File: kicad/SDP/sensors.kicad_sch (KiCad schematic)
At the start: 13 parts, among them J10 Limit, J11 Conn_01x07, J12 Conn_01x07, J13 Conn_01x03, J14 Conn_01x03, J8 Conn_01x07, J9 Conn_01x07

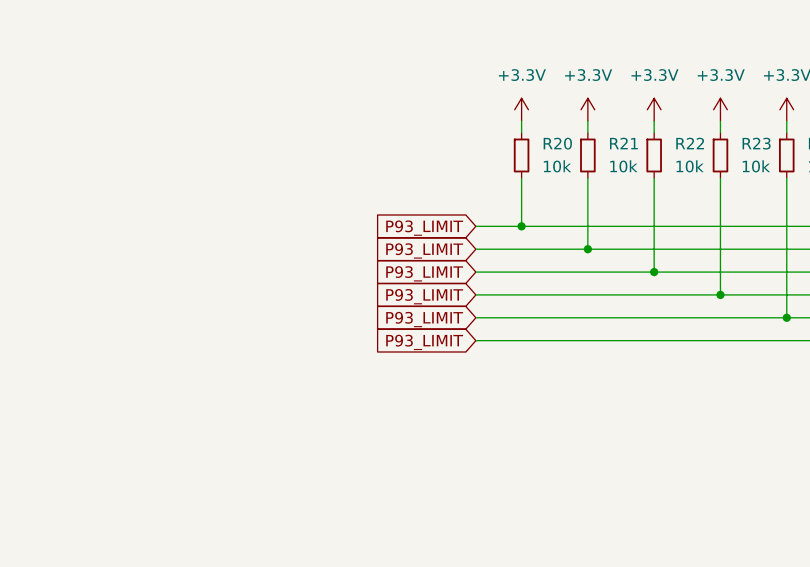
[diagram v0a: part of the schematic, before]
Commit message: PCB layout and schematic updates
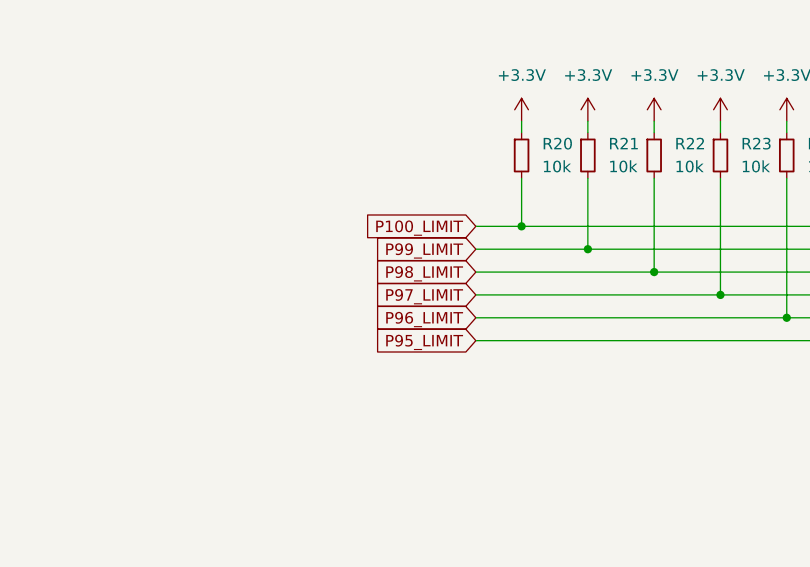
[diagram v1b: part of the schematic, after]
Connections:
- removed net P93_LIMIT: J10.1 (Pin_1), J10.11 (Pin_11), J10.3 (Pin_3), J10.5 (Pin_5), J10.7 (Pin_7), J10.9 (Pin_9), R20.2, R21.2, R22.2, R23.2, R24.2, R25.2
- new net P100_LIMIT: J10.1 (Pin_1), R20.2
- new net P95_LIMIT: J10.11 (Pin_11), R25.2
- new net P96_LIMIT: J10.9 (Pin_9), R24.2
- new net P97_LIMIT: J10.7 (Pin_7), R23.2
- new net P98_LIMIT: J10.5 (Pin_5), R22.2
- new net P99_LIMIT: J10.3 (Pin_3), R21.2
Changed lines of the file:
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@@
     (effects (font (size 1.27 1.27)) (justify left bottom))
+  )
+  (global_label "P100_LIMIT" (shape input) (at 179.832 53.086 180) (fields_autoplaced)
+    (effects (font (size 1.27 1.27)) (justify right))
+    (property "Intersheet References" "${INTERSHEET_REFS}" (id 0) (at 166.896 53.1654 0)
+      (effects (font (size 1.27 1.27)) (justify right) hide)
+    )
   )
   (global_label "P57_SCL1" (shape input) (at 91.694 39.116 180) (fields_autoplaced)
@@
     (effects (font (size 1.27 1.27)) (justify right))
     (property "Intersheet References" "${INTERSHEET_REFS}" (id 0) (at 73.3757 44.1166 0)
-      (effects (font (size 1.27 1.27)) (justify right) hide)
-    )
-  )
-  (global_label "P93_LIMIT" (shape input) (at 179.832 60.706 180) (fields_autoplaced)
-    (effects (font (size 1.27 1.27)) (justify right))
-    (property "Intersheet References" "${INTERSHEET_REFS}" (id 0) (at 168.1056 60.6266 0)
       (effects (font (size 1.27 1.27)) (justify right) hide)
     )
@@
     )
   )
+  (global_label "P95_LIMIT" (shape input) (at 179.832 65.786 180) (fields_autoplaced)
+    (effects (font (size 1.27 1.27)) (justify right))
+    (property "Intersheet References" "${INTERSHEET_REFS}" (id 0) (at 168.1056 65.7066 0)
+      (effects (font (size 1.27 1.27)) (justify right) hide)
+    )
+  )
   (global_label "P56_SDA1" (shape input) (at 91.694 36.576 180) (fields_autoplaced)
     (effects (font (size 1.27 1.27)) (justify right))
     (property "Intersheet References" "${INTERSHEET_REFS}" (id 0) (at 79.8466 36.4966 0)
+      (effects (font (size 1.27 1.27)) (justify right) hide)
+    )
+  )
+  (global_label "P97_LIMIT" (shape input) (at 179.832 60.706 180) (fields_autoplaced)
+    (effects (font (size 1.27 1.27)) (justify right))
+    (property "Intersheet References" "${INTERSHEET_REFS}" (id 0) (at 168.1056 60.6266 0)
       (effects (font (size 1.27 1.27)) (justify right) hide)
     )
@@
     )
   )
-  (global_label "P93_LIMIT" (shape input) (at 179.832 63.246 180) (fields_autoplaced)
+  (global_label "P96_LIMIT" (shape input) (at 179.832 63.246 180) (fields_autoplaced)
     (effects (font (size 1.27 1.27)) (justify right))
     (property "Intersheet References" "${INTERSHEET_REFS}" (id 0) (at 168.1056 63.1666 0)
+      (effects (font (size 1.27 1.27)) (justify right) hide)
+    )
+  )
+  (global_label "P99_LIMIT" (shape input) (at 179.832 55.626 180) (fields_autoplaced)
+    (effects (font (size 1.27 1.27)) (justify right))
+    (property "Intersheet References" "${INTERSHEET_REFS}" (id 0) (at 168.1056 55.7054 0)
       (effects (font (size 1.27 1.27)) (justify right) hide)
     )
@@
     )
   )
+  (global_label "P98_LIMIT" (shape input) (at 179.832 58.166 180) (fields_autoplaced)
+    (effects (font (size 1.27 1.27)) (justify right))
+    (property "Intersheet References" "${INTERSHEET_REFS}" (id 0) (at 168.1056 58.2454 0)
+      (effects (font (size 1.27 1.27)) (justify right) hide)
+    )
+  )
   (global_label "P57_SCL1" (shape input) (at 91.694 72.39 180) (fields_autoplaced)
     (effects (font (size 1.27 1.27)) (justify right))
     (property "Intersheet References" "${INTERSHEET_REFS}" (id 0) (at 79.9071 72.3106 0)
-      (effects (font (size 1.27 1.27)) (justify right) hide)
-    )
-  )
-  (global_label "P93_LIMIT" (shape input) (at 179.832 58.166 180) (fields_autoplaced)
-    (effects (font (size 1.27 1.27)) (justify right))
-    (property "Intersheet References" "${INTERSHEET_REFS}" (id 0) (at 168.1056 58.0866 0)
-      (effects (font (size 1.27 1.27)) (justify right) hide)
-    )
-  )
-  (global_label "P93_LIMIT" (shape input) (at 179.832 55.626 180) (fields_autoplaced)
-    (effects (font (size 1.27 1.27)) (justify right))
-    (property "Intersheet References" "${INTERSHEET_REFS}" (id 0) (at 168.1056 55.5466 0)
       (effects (font (size 1.27 1.27)) (justify right) hide)
     )
@@
       (effects (font (size 1.27 1.27)) (justify right) hide)
     )
-  )
-  (global_label "P93_LIMIT" (shape input) (at 179.832 65.786 180) (fields_autoplaced)
-    (effects (font (size 1.27 1.27)) (justify right))
-    (property "Intersheet References" "${INTERSHEET_REFS}" (id 0) (at 168.1056 65.7066 0)
-      (effects (font (size 1.27 1.27)) (justify right) hide)
-    )
-  )
-  (global_label "P93_LIMIT" (shape input) (at 179.832 53.086 180) (fields_autoplaced)
-    (effects (font (size 1.27 1.27)) (justify right))
-    (property "Intersheet References" "${INTERSHEET_REFS}" (id 0) (at 168.1056 53.0066 0)
-      (effects (font (size 1.27 1.27)) (justify right) hide)
-    )

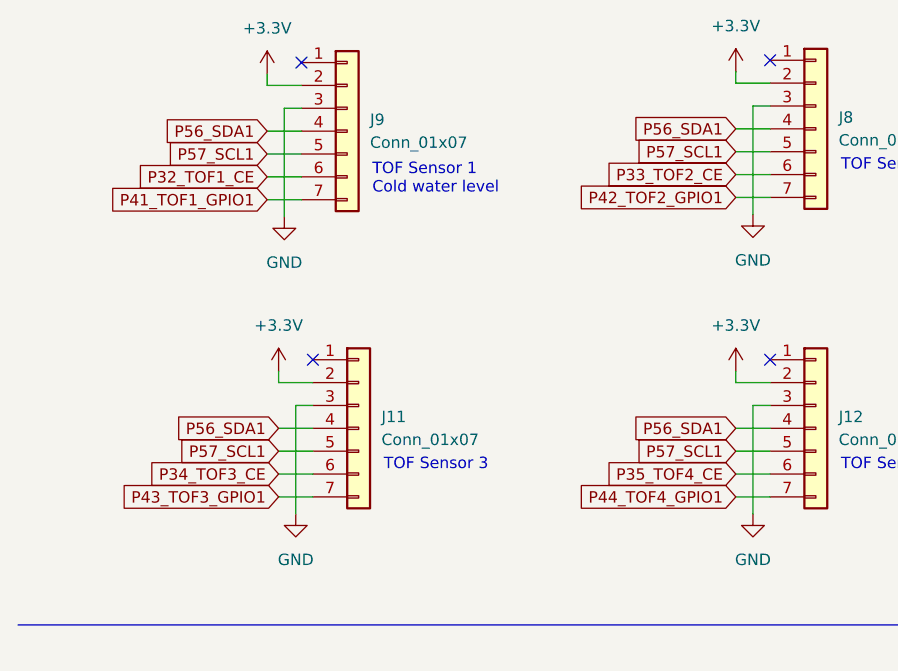
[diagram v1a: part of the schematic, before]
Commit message: Controller PCB layout
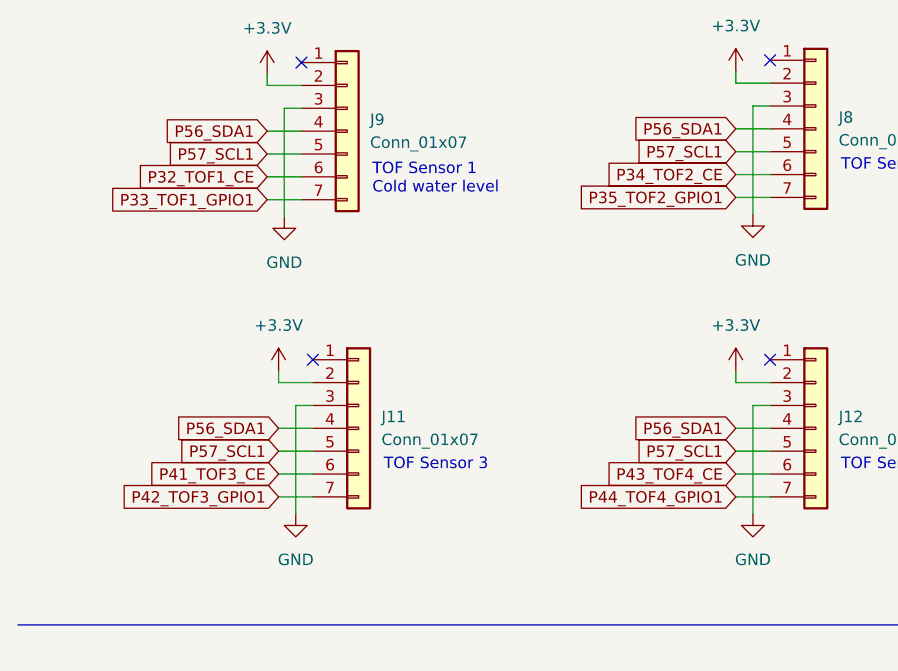
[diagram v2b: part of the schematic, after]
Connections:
- net P33_TOF2_CE renamed P34_TOF2_CE
- net P34_TOF3_CE renamed P41_TOF3_CE
- net P35_TOF4_CE renamed P43_TOF4_CE
- net P41_TOF1_GPIO1 renamed P33_TOF1_GPIO1
- net P42_TOF2_GPIO1 renamed P35_TOF2_GPIO1
- net P43_TOF3_GPIO1 renamed P42_TOF3_GPIO1
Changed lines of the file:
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@@
     )
   )
-  (global_label "P42_TOF2_GPIO1" (shape input) (at 91.694 44.196 180) (fields_autoplaced)
+  (global_label "P35_TOF2_GPIO1" (shape input) (at 91.694 44.196 180) (fields_autoplaced)
     (effects (font (size 1.27 1.27)) (justify right))
     (property "Intersheet References" "${INTERSHEET_REFS}" (id 0) (at 73.3757 44.1166 0)
@@
     )
   )
-  (global_label "P34_TOF3_CE" (shape input) (at 40.894 74.93 180) (fields_autoplaced)
+  (global_label "P41_TOF3_CE" (shape input) (at 40.894 74.93 180) (fields_autoplaced)
     (effects (font (size 1.27 1.27)) (justify right))
     (property "Intersheet References" "${INTERSHEET_REFS}" (id 0) (at 25.8414 74.8506 0)
@@
     )
   )
-  (global_label "P43_TOF3_GPIO1" (shape input) (at 40.894 77.47 180) (fields_autoplaced)
+  (global_label "P42_TOF3_GPIO1" (shape input) (at 40.894 77.47 180) (fields_autoplaced)
     (effects (font (size 1.27 1.27)) (justify right))
     (property "Intersheet References" "${INTERSHEET_REFS}" (id 0) (at 22.5757 77.3906 0)
@@
     )
   )
-  (global_label "P35_TOF4_CE" (shape input) (at 91.694 74.93 180) (fields_autoplaced)
+  (global_label "P43_TOF4_CE" (shape input) (at 91.694 74.93 180) (fields_autoplaced)
     (effects (font (size 1.27 1.27)) (justify right))
     (property "Intersheet References" "${INTERSHEET_REFS}" (id 0) (at 76.6414 74.8506 0)
@@
     )
   )
-  (global_label "P41_TOF1_GPIO1" (shape input) (at 39.624 44.45 180) (fields_autoplaced)
+  (global_label "P33_TOF1_GPIO1" (shape input) (at 39.624 44.45 180) (fields_autoplaced)
     (effects (font (size 1.27 1.27)) (justify right))
     (property "Intersheet References" "${INTERSHEET_REFS}" (id 0) (at 21.3057 44.3706 0)
@@
     )
   )
-  (global_label "P33_TOF2_CE" (shape input) (at 91.694 41.656 180) (fields_autoplaced)
+  (global_label "P34_TOF2_CE" (shape input) (at 91.694 41.656 180) (fields_autoplaced)
     (effects (font (size 1.27 1.27)) (justify right))
     (property "Intersheet References" "${INTERSHEET_REFS}" (id 0) (at 76.6414 41.5766 0)
